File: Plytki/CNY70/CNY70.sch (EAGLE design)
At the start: 5 parts

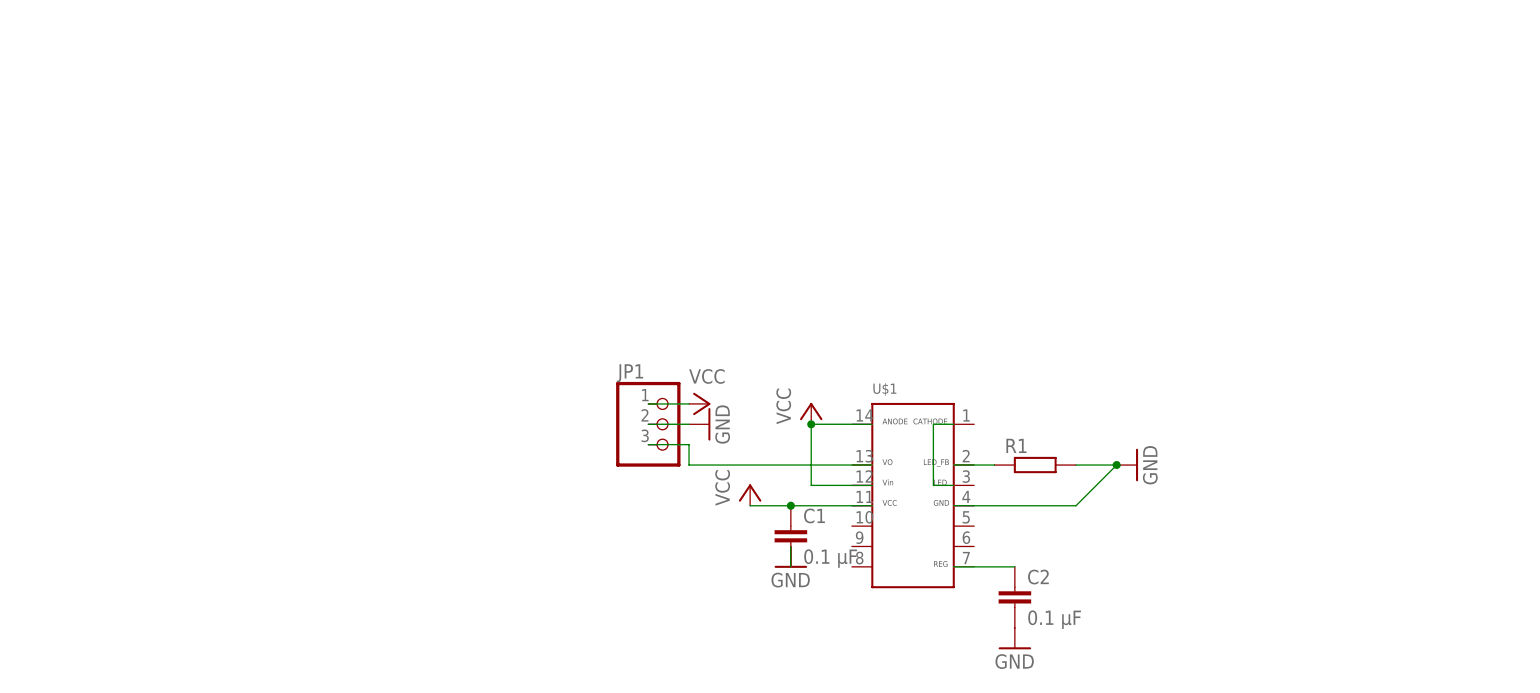
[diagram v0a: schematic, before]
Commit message: Ostateczne projekty plytek
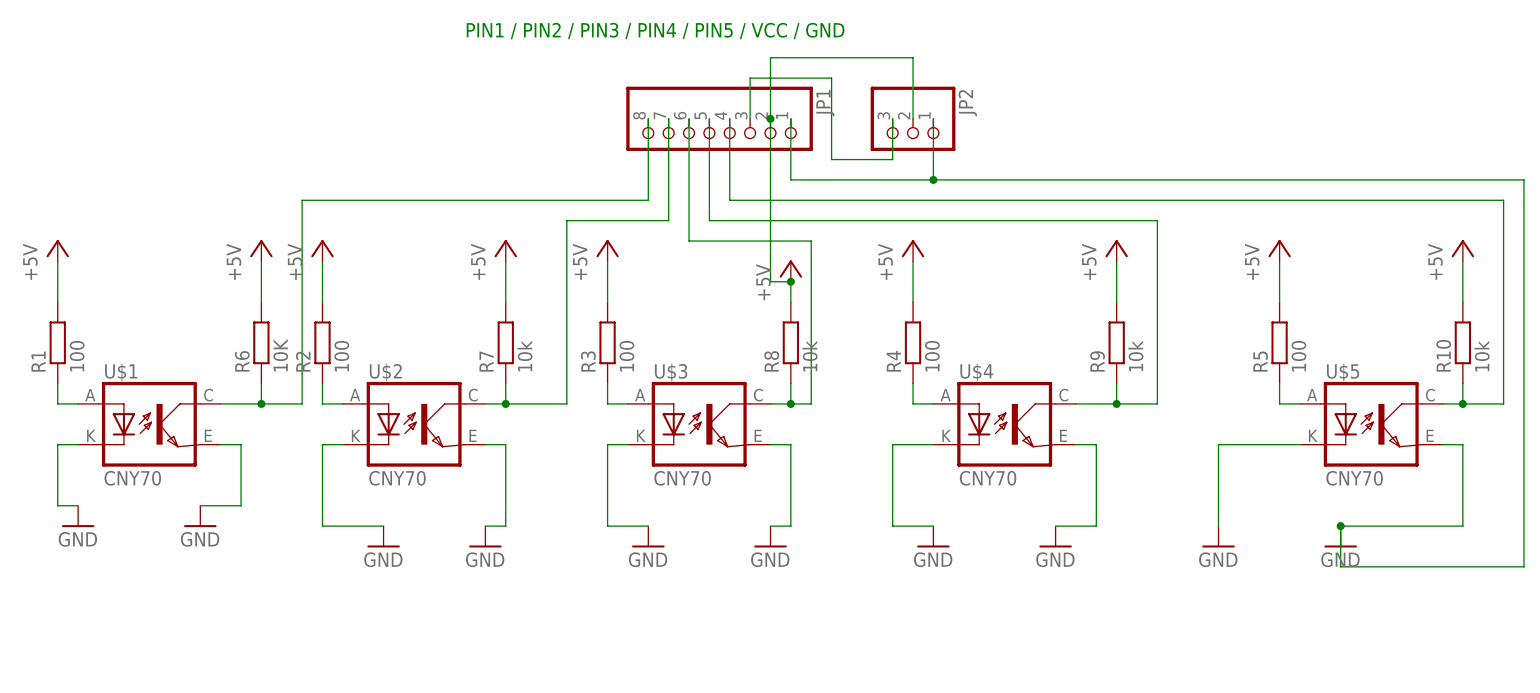
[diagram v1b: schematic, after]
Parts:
- removed C1, C2: 0.1 μF, rcl:C-EU025-025X050
- added JP2: (no value), pinhead:PINHD-1X3
- added R10, R7, R8, R9: 10k, rcl:R-EU_0309/12
- added R2, R3, R4, R5: 100, rcl:R-EU_0309/12
- added R6: 10K, rcl:R-EU_0309/12
- added U$2, U$3, U$4, U$5: CNY70, cny70:CNY70
- JP1: device pinhead:PINHD-1X3 -> pinhead:PINHD-1X8
- R1: value (none) -> 100; device rcl:R-EU_0204/5 -> rcl:R-EU_0309/12
- U$1: value SHARP-DIST -> CNY70; device sharp-dist:SHARP-DIST -> cny70:CNY70
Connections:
- removed net VCC: C1.1, JP1.1, U$1.11, U$1.12, U$1.14
- new net +5V: JP1.2, JP2.2, R1.2, R10.2, R2.2, R3.2, R4.2, R5.2, R6.2, R7.2, R8.2, R9.2
- new net N$10: JP1.4, R10.1, U$5.COL
- new net N$12: JP1.5, R9.1, U$4.COL
- new net N$5: R5.1, U$5.A
- new net N$6: JP1.8, R6.1, U$1.COL
- new net N$7: JP1.7, R7.1, U$2.COL
- new net N$8: JP1.6, R8.1, U$3.COL
- new net N$9: JP1.3, JP2.3
- net GND: now also JP1.1, JP2.1, U$1.C, U$1.EMI, U$2.C, U$2.EMI, U$3.C, U$3.EMI, U$4.C, U$4.EMI, U$5.C, U$5.EMI; no longer C1.2, C2.2, JP1.2, R1.2, U$1.4
- net N$1: now also R1.1, U$1.A; no longer U$1.1, U$1.3
- net N$2: now also R2.1, U$2.A; no longer R1.1, U$1.2
- net N$3: now also R3.1, U$3.A; no longer C2.1, U$1.7
- net N$4: now also R4.1, U$4.A; no longer JP1.3, U$1.13
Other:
- note added: "PIN1 / PIN2 / PIN3 / PIN4 / PIN5 / VCC / GND"
- moved on the sheet: R1
